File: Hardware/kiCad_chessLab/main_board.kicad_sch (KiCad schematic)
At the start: 41 parts, among them Q1 CH221K, SW2 RST, SW3 BOOT, U1 ESP32-S3-WROOM-1, U12 TP5100_C379389, U2 USB-TYPE-C-019, U3 74HC138

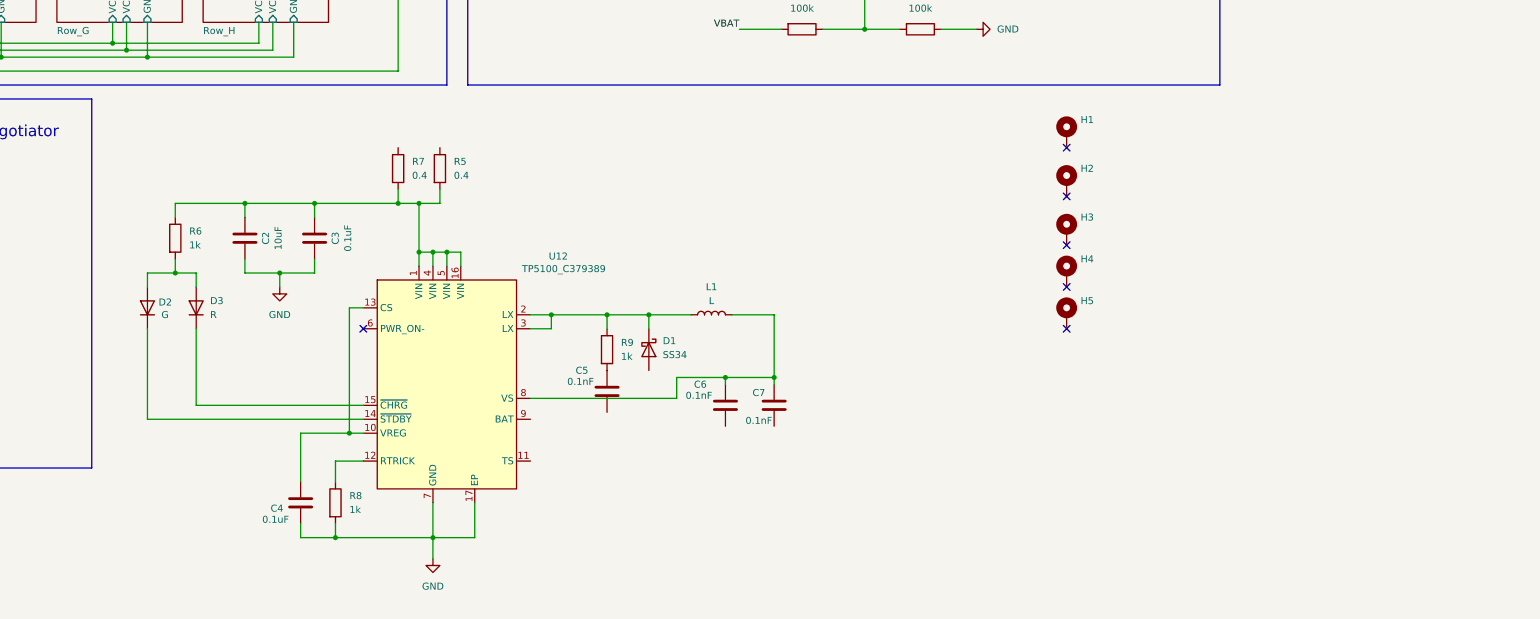
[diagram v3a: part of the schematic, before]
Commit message: save
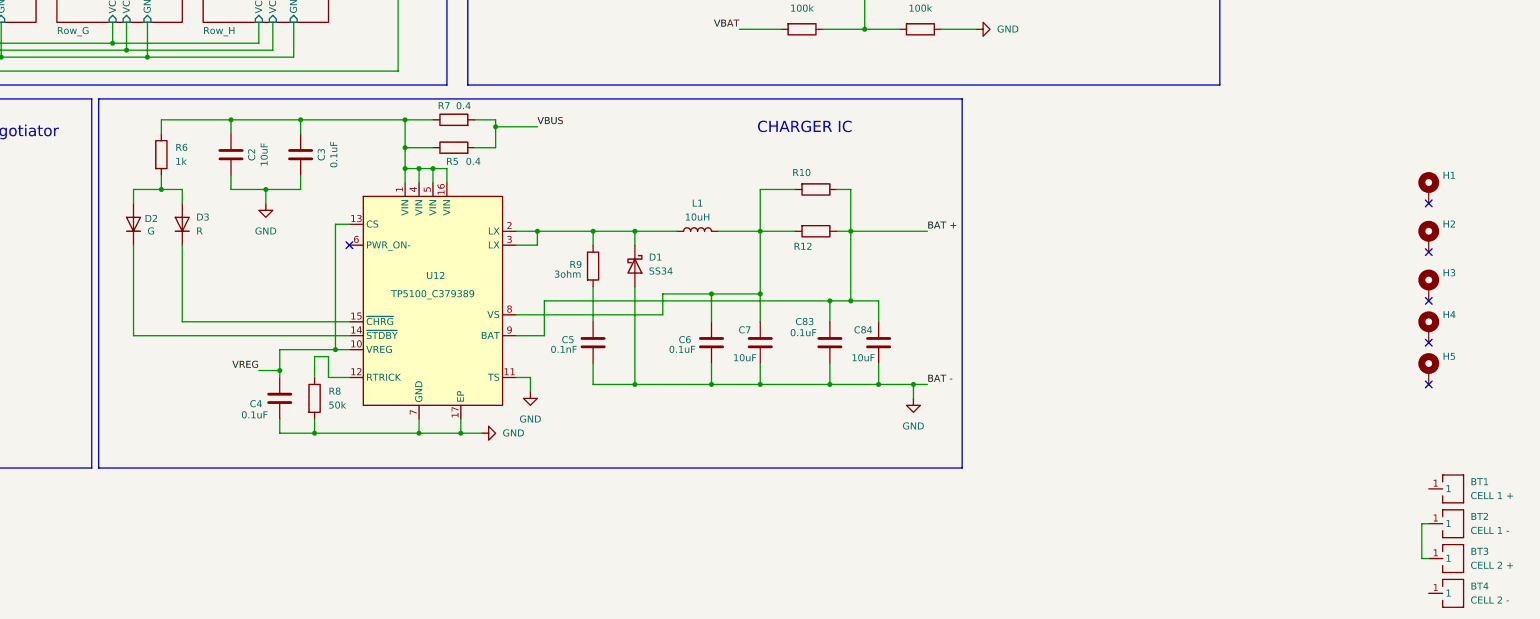
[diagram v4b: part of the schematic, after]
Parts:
- added BT1: CELL 1 +, chessLab-footprints:BAT-TH_MY-18650-01, symbol chessLab-symbols:MY-18650-01
- added BT2: CELL 1 -, chessLab-footprints:BAT-TH_MY-18650-01, symbol chessLab-symbols:MY-18650-01
- added BT3: CELL 2 +, chessLab-footprints:BAT-TH_MY-18650-01, symbol chessLab-symbols:MY-18650-01
- added BT4: CELL 2 -, chessLab-footprints:BAT-TH_MY-18650-01, symbol chessLab-symbols:MY-18650-01
- added C83: 0.1uF, Capacitor_SMD:C_0603_1608Metric_Pad1.08x0.95mm_HandSolder, symbol Device:C
- added C84: 10uF, Capacitor_SMD:C_1210_3225Metric_Pad1.33x2.70mm_HandSolder, symbol Device:C
- added R10, R12: 0,1, Resistor_SMD:R_1206_3216Metric_Pad1.30x1.75mm_HandSolder, symbol Device:R
- C2: footprint Capacitor_SMD:C_0201_0603Metric_Pad0.64x0.40mm_HandSolder -> Capacitor_SMD:C_1210_3225Metric_Pad1.33x2.70mm_HandSolder
- C3, C4, C5: footprint Capacitor_SMD:C_0201_0603Metric_Pad0.64x0.40mm_HandSolder -> Capacitor_SMD:C_0603_1608Metric_Pad1.08x0.95mm_HandSolder
- C6: value 0.1nF -> 0.1uF; footprint Capacitor_SMD:C_0201_0603Metric_Pad0.64x0.40mm_HandSolder -> Capacitor_SMD:C_0603_1608Metric_Pad1.08x0.95mm_HandSolder
- C7: value 0.1nF -> 10uF; footprint Capacitor_SMD:C_0201_0603Metric_Pad0.64x0.40mm_HandSolder -> Capacitor_SMD:C_1210_3225Metric_Pad1.33x2.70mm_HandSolder
- L1: value L -> 10uH; footprint (none) -> Inductor_SMD:L_TechFuse_SL0520
- R8: value 1k -> 50k
- R9: value 1k -> 3ohm
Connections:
- net GND: now also C5.1, C6.1, C7.1, D1.2 (A), U12.11 (TS), C83.1, C84.1
- net VBUS: now also R5.2, R7.2
- net at R5.1: now also C2.2, C3.2, R6.1, R7.1, U12.1 (VIN), U12.16 (VIN), U12.4 (VIN), U12.5 (VIN)
- net at C6.2, C7.2, L1.2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: now also R10.2, R12.2
- net VREG: now reaches C4.2, U12.10 (VREG), U12.13 (CS)
- net BAT +: now reaches U12.9 (BAT)
- net BAT +: now also C83.2, C84.2, R10.1, R12.1
- new net: BT2.1, BT3.1
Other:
- note added: "CHARGER IC"
- moved on the sheet: C2, C3, C4, C5, C6, C7, D1, D2, D3, H1, H2, H3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
